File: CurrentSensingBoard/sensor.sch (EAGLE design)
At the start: 13 parts, among them U1 MAX11634EEE+T21-0055H_16-L

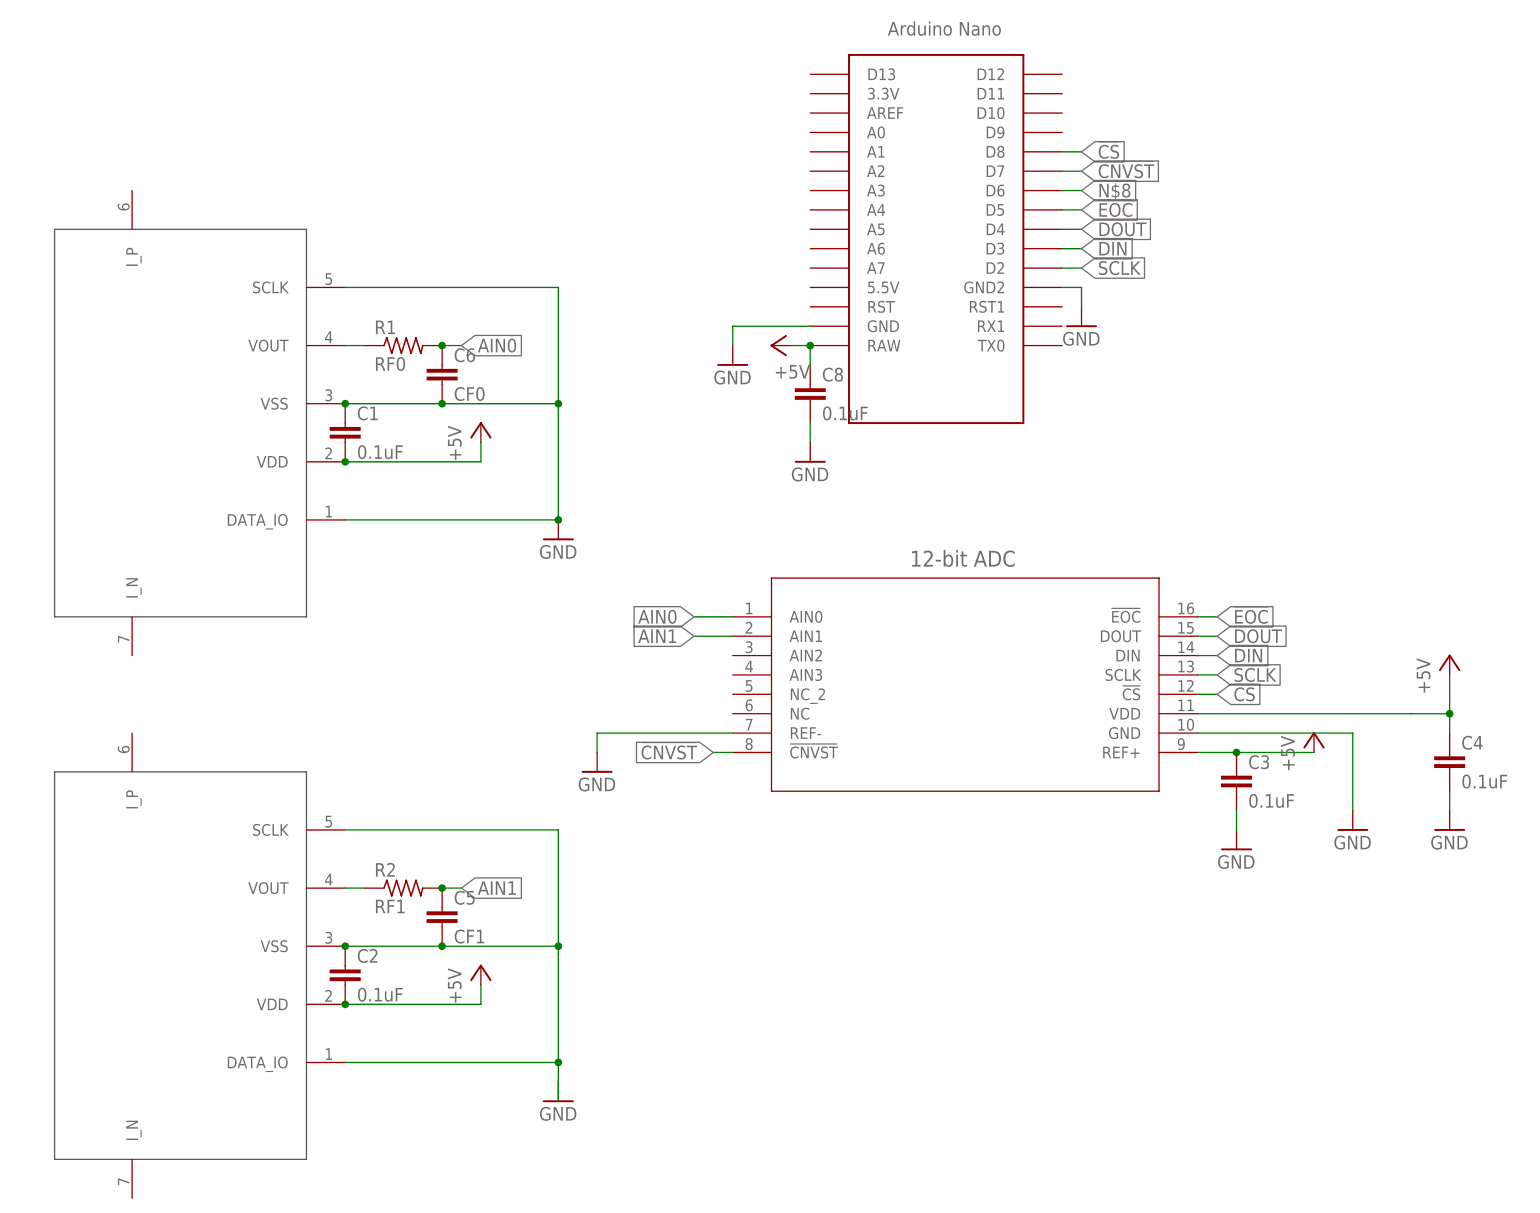
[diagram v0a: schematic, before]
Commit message: finished schem for reals
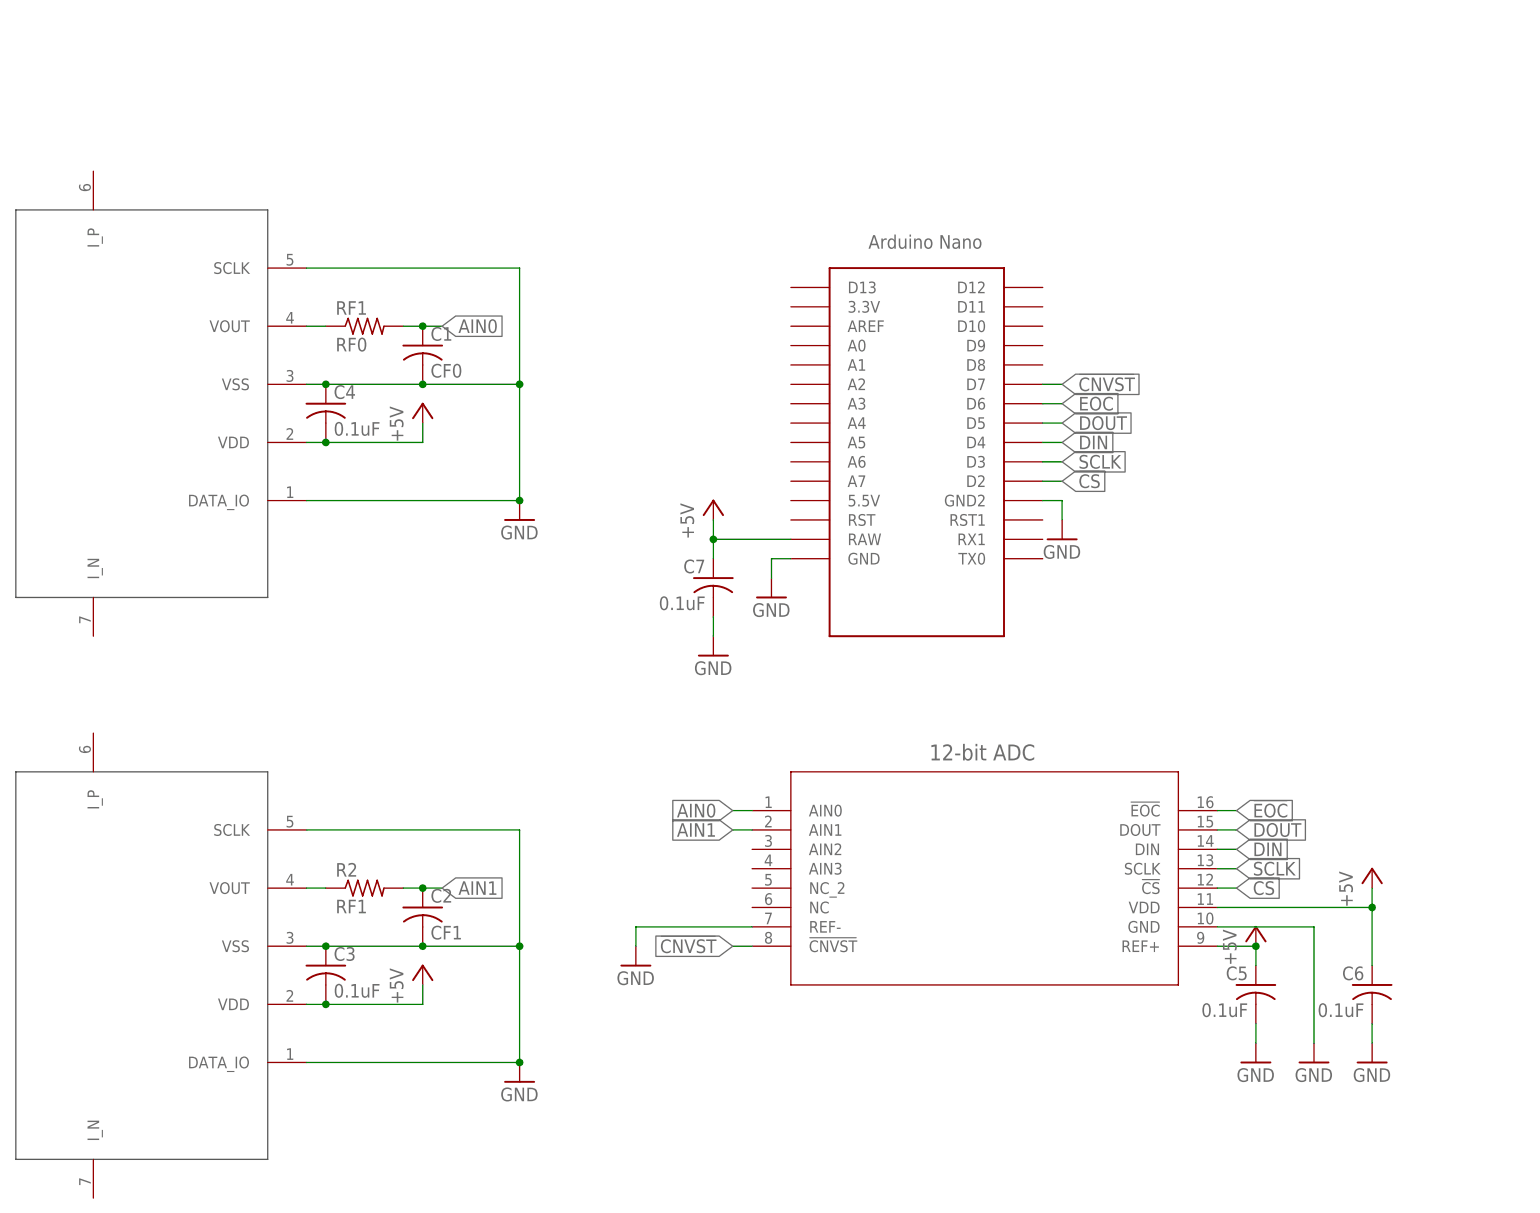
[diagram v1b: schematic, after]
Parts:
- removed C8: 0.1uF, SparkFun-Capacitors:0.1UF-0603-100V-10%
- removed R1: RF0, rcl:R-US_R0603
- added C7: 0.1uF, rcl:C-USC0603
- added RF1: RF0, rcl:R-US_R0603
- C1: value 0.1uF -> CF0; device SparkFun-Capacitors:0.1UF-0603-100V-10% -> rcl:C-USC0603
- C2: value 0.1uF -> CF1; device SparkFun-Capacitors:0.1UF-0603-100V-10% -> rcl:C-USC0603
- C3, C4: device SparkFun-Capacitors:0.1UF-0603-100V-10% -> rcl:C-USC0603
- C5: value CF1 -> 0.1uF; device SparkFun-Capacitors:0.1UF-0603-100V-10% -> rcl:C-USC0603
- C6: value CF0 -> 0.1uF; device SparkFun-Capacitors:0.1UF-0603-100V-10% -> rcl:C-USC0603
- U$1: value CQ2065 -> NANO; device CurrentSensing:CQ2065 -> I'mRADIOactive:NANO
- U$3: value NANO -> CQ2065; device I'mRADIOactive:NANO -> CurrentSensing:CQ2065
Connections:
- removed net N$4: R2.1, U$2.VOUT
- removed net N$8: U$3.D6
- removed net VDD: C4.1, U1.VDD
- new net N$5: RF1.1, U$2.VOUT
- net !CNVST!: now also U$1.D7; no longer U$3.D7
- net !CS!: now also U$1.D2; no longer U$3.D8
- net !EOC!: now also U$1.D6; no longer U$3.D5
- net +5V: now also C3.2, C4.2, C5.1, C6.1, C7.1, U$1.RAW, U$3.VDD, U1.VDD; no longer C1.2, C2.2, C3.1, C8.1, U$1.VDD, U$3.RAW
- net AIN0: now also C1.1, RF1.2; no longer C6.1, R1.2
- net AIN1: now also C2.1; no longer C5.1
- net DIN: now also U$1.D4; no longer U$3.D3
- net DOUT: now also U$1.D5; no longer U$3.D4
- net GND: now also C1.2, C2.2, C3.1, C4.1, C7.2, U$1.GND, U$1.GND2, U$3.DATA_IO, U$3.SCLK, U$3.VSS; no longer C1.1, C2.1, C3.2, C4.2, C8.2, U$1.DATA_IO, U$1.SCLK, U$1.VSS, U$3.GND, U$3.GND2
- net N$3: now also R2.1, U$3.VOUT; no longer R1.1, U$1.VOUT
- net SCLK: now also U$1.D3; no longer U$3.D2
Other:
- moved on the sheet: C1, C2, C3, C4, C5, C6, R2
